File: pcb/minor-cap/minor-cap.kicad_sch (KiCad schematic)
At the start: 25 parts, among them J1 Conn_01x17, SW1 SW_SPDT, U1 QT60160, U2 keys, U3 keys, U4 ATtiny1614-SS, U6 MCP6001R

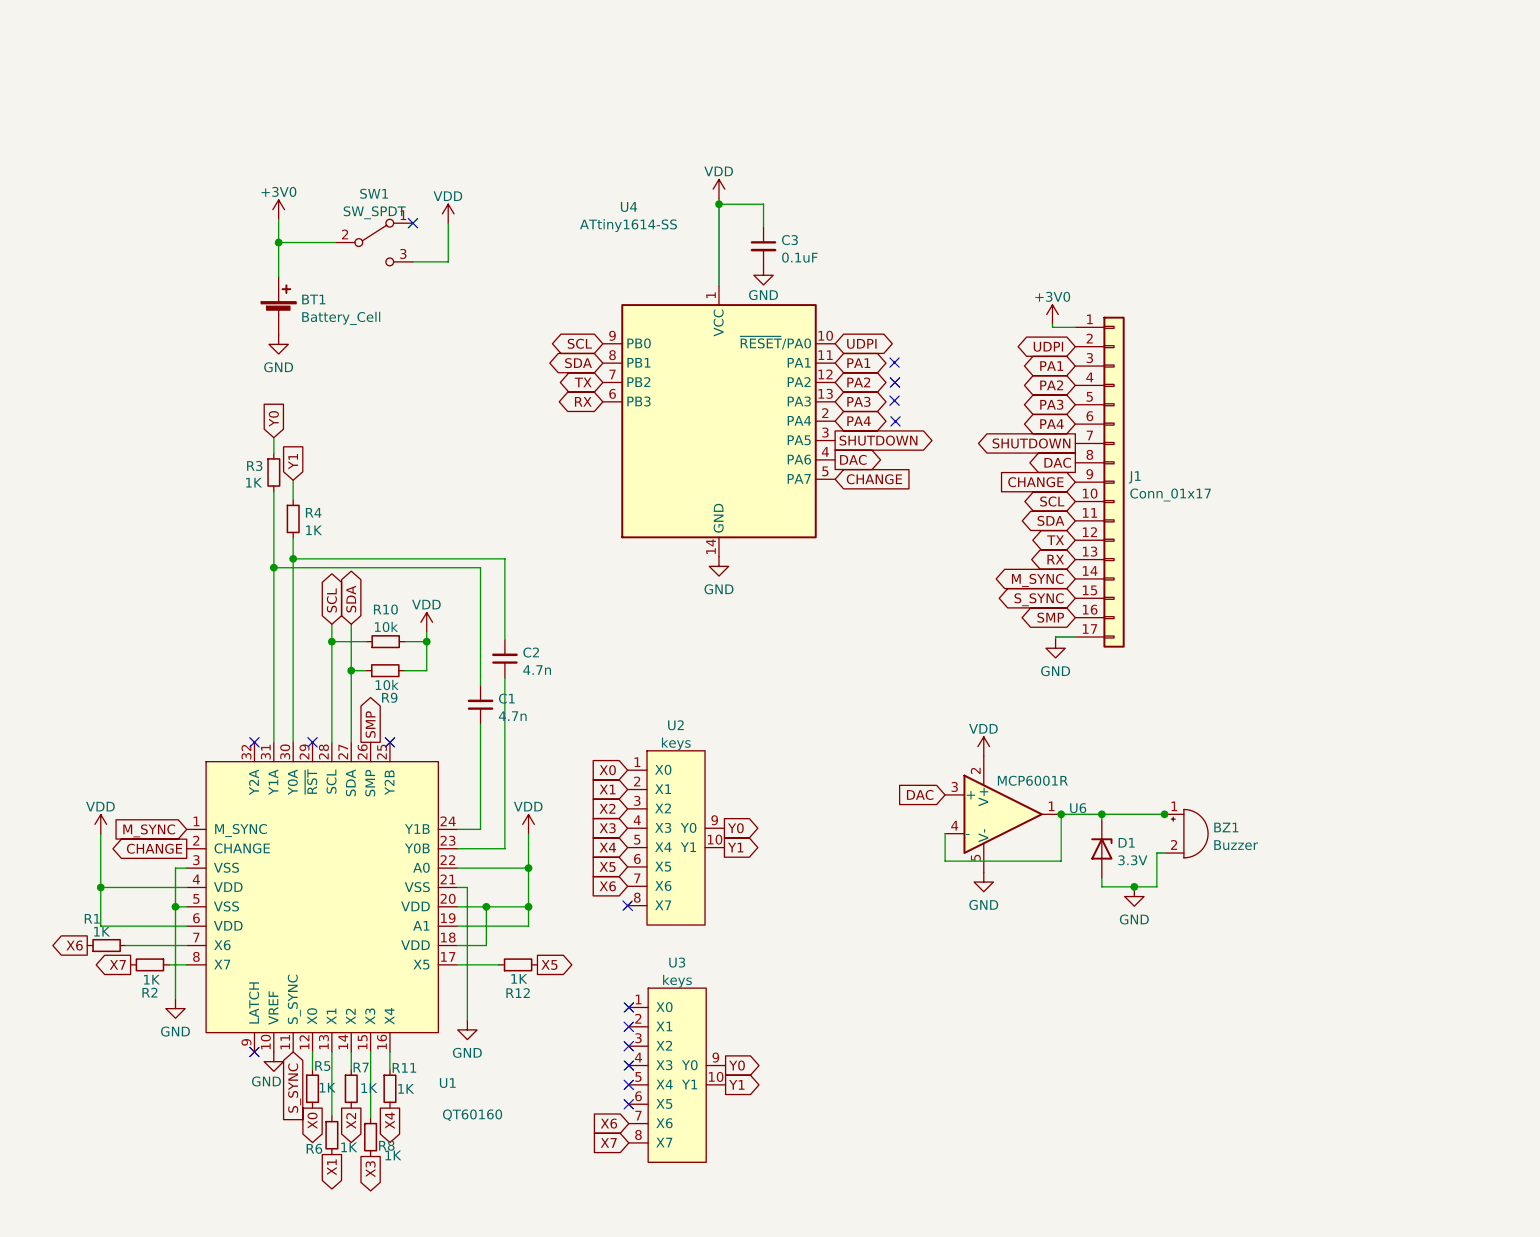
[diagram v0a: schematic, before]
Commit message: routed
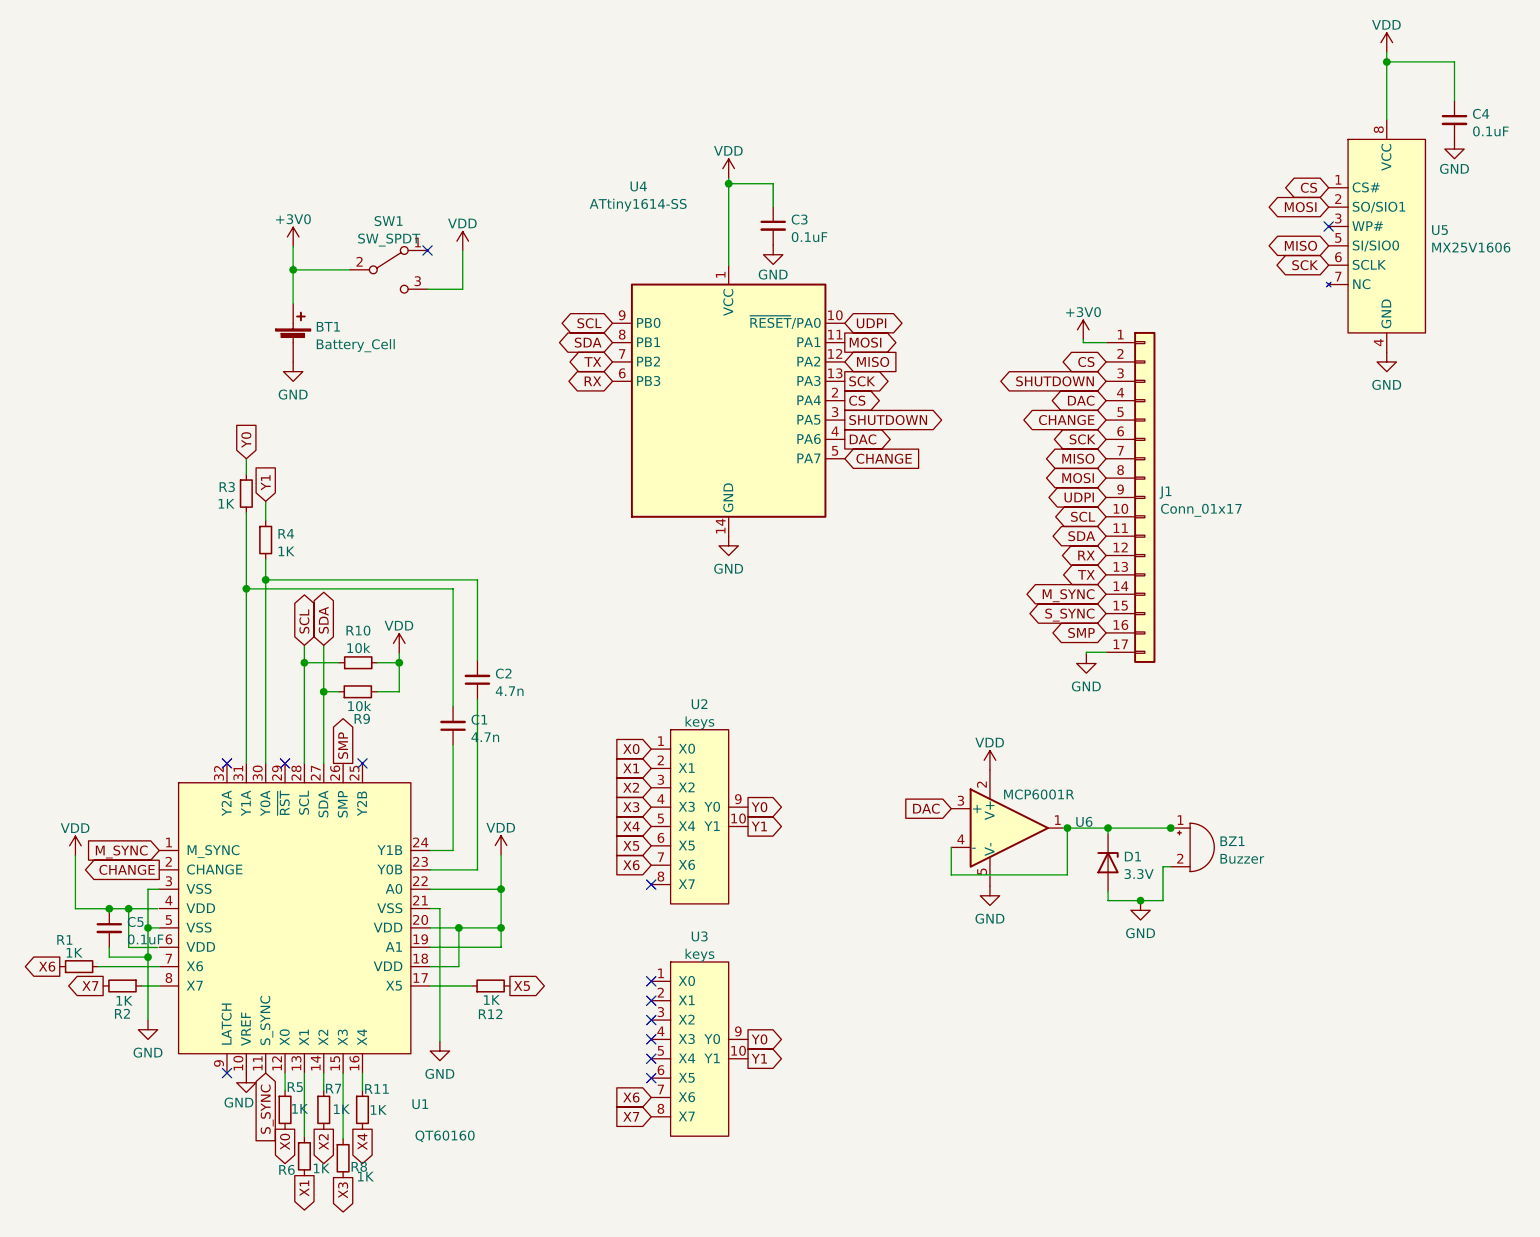
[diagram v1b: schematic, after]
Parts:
- added C4, C5: 0.1uF, Capacitor_SMD:C_0603_1608Metric, symbol Device:C_Small
- added U5: MX25V1606, Package_SO:SOP-8_3.9x4.9mm_P1.27mm, symbol MX25V1606:MX25V1606
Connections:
- net CHANGE: now also J1.5 (Pin_5); no longer J1.9 (Pin_9)
- net DAC: now also J1.4 (Pin_4); no longer J1.8 (Pin_8)
- net GND: now also C4.2, C5.2, U5.4 (GND)
- net RX: now also J1.12 (Pin_12); no longer J1.13 (Pin_13)
- net SHUTDOWN: now also J1.3 (Pin_3); no longer J1.7 (Pin_7)
- net TX: now also J1.13 (Pin_13); no longer J1.12 (Pin_12)
- net UDPI: now also J1.9 (Pin_9); no longer J1.2 (Pin_2)
- net VDD: now also C4.1, C5.1, U5.8 (VCC); no longer U1.4 (VDD), U1.6 (VDD)
- net PA1 renamed MOSI
- net MOSI: now also J1.8 (Pin_8), U5.2 (SO/SIO1); no longer J1.3 (Pin_3)
- net PA2 renamed MISO
- net MISO: now also J1.7 (Pin_7), U5.5 (SI/SIO0); no longer J1.4 (Pin_4)
- net PA3 renamed SCK
- net SCK: now also J1.6 (Pin_6), U5.6 (SCLK); no longer J1.5 (Pin_5)
- net PA4 renamed CS
- net CS: now also J1.2 (Pin_2), U5.1 (CS#); no longer J1.6 (Pin_6)
- no-connect marks 16 -> 13
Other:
- moved on the sheet: BT1, BZ1, C1, C2, C3, D1, J1, R1, R10, R11, R12, R2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

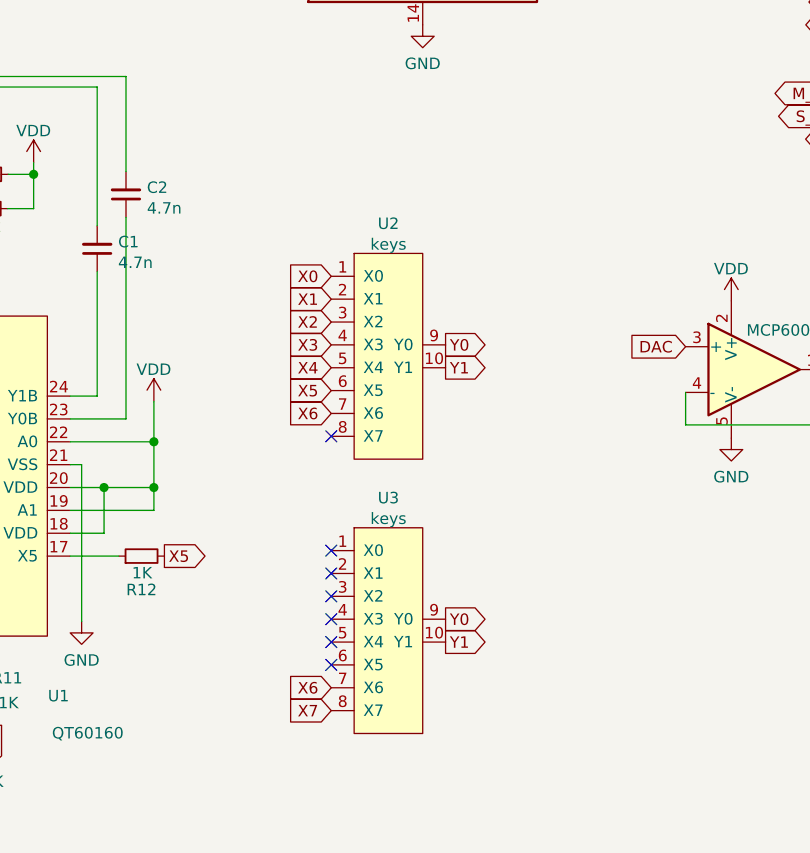
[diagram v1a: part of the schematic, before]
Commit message: routed
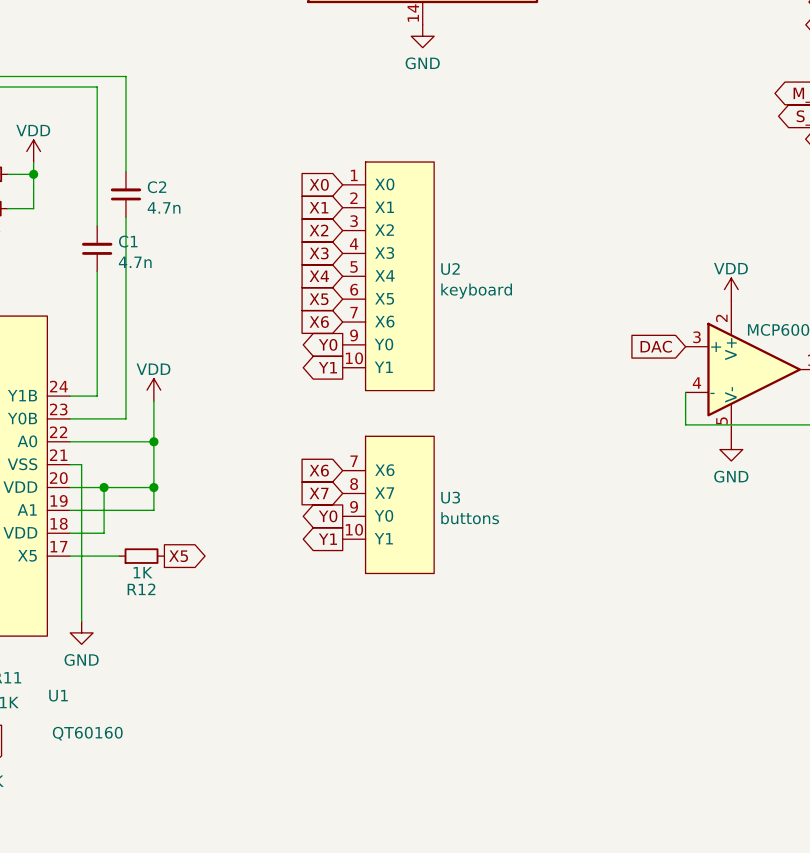
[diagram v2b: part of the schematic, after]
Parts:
- removed U2: keys, keys:13-keys, symbol keyboard-13:keys
- removed U3: keys, keys:3-buttons, symbol keyboard-13:keys
- added U2: keyboard, keys:13-keys, symbol keyboard-13:keyboard
- added U3: buttons, keys:3-buttons, symbol keyboard-13:buttons
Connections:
- net X0: now also U2.1 (X0)
- net X1: now also U2.2 (X1)
- net X2: now also U2.3 (X2)
- net X3: now also U2.4 (X3)
- net X4: now also U2.5 (X4)
- net X5: now also U2.6 (X5)
- net X6: now also U2.7 (X6), U3.7 (X6)
- net X7: now also U3.8 (X7)
- net Y0: now also U2.9 (Y0), U3.9 (Y0)
- net Y1: now also U2.10 (Y1), U3.10 (Y1)
- no-connect marks 13 -> 6
